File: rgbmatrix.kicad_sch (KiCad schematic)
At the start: 134 parts

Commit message: fked up LEDs :C
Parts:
- D10, D11, D12, D13, D14, D15, D16, D17, D18, D19, D2, D20, D21, D22, D23, D24, D25, D26, D27, D28, D29, D3, D30, D31, D32, D33, D34, D35, D36, D37, D38, D39, D4, D40, D41, D42, D43, D44, D45, D46, D47, D48, D49, D5, D50, D51, D52, D53, D54, D55, D56, D57, D58, D59, D6, D60, D61, D62, D63, D64, D65, D66, D67, D68, D7, D8, D9: footprint LED_SMD:LED_SK6812MINI_PLCC4_3.5x3.5mm_P1.75mm -> reverse:MX_SK6812MINI-E_REV

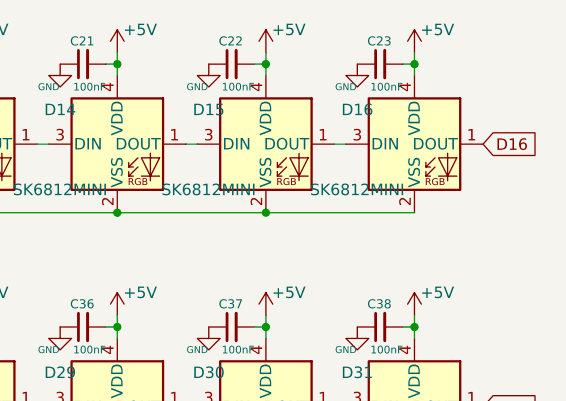
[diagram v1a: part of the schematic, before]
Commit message: pensive
changed LEDs aaaAAAAAAA
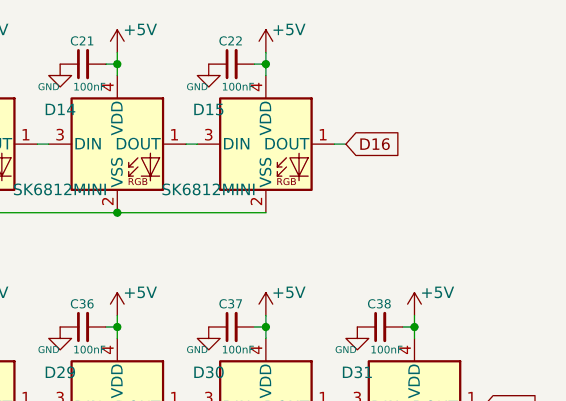
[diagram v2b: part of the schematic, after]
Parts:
- removed C23: 100nF, Capacitor_SMD:C_0805_2012Metric_Pad1.18x1.45mm_HandSolder, symbol Device:C_Small
- removed D16: SK6812MINI, reverse:MX_SK6812MINI-E_REV, symbol LED:SK6812MINI
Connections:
- net D16: now also D15.1 (DOUT)
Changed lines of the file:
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@@
   (junction (at 214.63 105.41) (diameter 0) (color 0 0 0 0)
   )
-  (junction (at 247.65 40.64) (diameter 0) (color 0 0 0 0)
-  )
   (junction (at 66.04 69.85) (diameter 0) (color 0 0 0 0)
   )
@@
   (junction (at 231.14 24.13) (diameter 0) (color 0 0 0 0)
   )
-  (junction (at 264.16 24.13) (diameter 0) (color 0 0 0 0)
-  )
   (junction (at 132.08 96.52) (diameter 0) (color 0 0 0 0)
   )
@@
     (stroke (width 0) (type default) (color 0 0 0 0))
   )
-  (wire (pts (xy 264.16 24.13) (xy 264.16 25.4))
-    (stroke (width 0) (type default) (color 0 0 0 0))
-  )
   (wire (pts (xy 49.53 22.86) (xy 49.53 24.13))
     (stroke (width 0) (type default) (color 0 0 0 0))
@@
     (stroke (width 0) (type default) (color 0 0 0 0))
   )
-  (wire (pts (xy 247.65 40.64) (xy 264.16 40.64))
-    (stroke (width 0) (type default) (color 0 0 0 0))
-  )
   (wire (pts (xy 198.12 80.01) (xy 198.12 81.28))
     (stroke (width 0) (type default) (color 0 0 0 0))
@@
     (stroke (width 0) (type default) (color 0 0 0 0))
   )
-  (wire (pts (xy 264.16 22.86) (xy 264.16 24.13))
-    (stroke (width 0) (type default) (color 0 0 0 0))
-  )
   (wire (pts (xy 148.59 69.85) (xy 165.1 69.85))
     (stroke (width 0) (type default) (color 0 0 0 0))
@@
     (stroke (width 0) (type default) (color 0 0 0 0))
   )
-  (wire (pts (xy 262.89 24.13) (xy 264.16 24.13))
-    (stroke (width 0) (type default) (color 0 0 0 0))
-  )
   (wire (pts (xy 165.1 69.85) (xy 181.61 69.85))
     (stroke (width 0) (type default) (color 0 0 0 0))
@@
     )
   )
-  (global_label "D16" (shape input) (at 271.78 33.02 0) (fields_autoplaced)
+  (global_label "D16" (shape input) (at 256.54 33.02 0) (fields_autoplaced)
     (effects (font (size 1.27 1.27)) (justify left))
-    (property "Intersheet References" "${INTERSHEET_REFS}" (id 0) (at 277.8821 32.9406 0)
+    (property "Intersheet References" "${INTERSHEET_REFS}" (id 0) (at 262.6421 32.9406 0)
       (effects (font (size 1.27 1.27)) (justify left) hide)
     )
@@
     (pin "2")
   )
-  (symbol (lib_id "Device:C_Small") (at 260.35 24.13 90) (unit 1)
-    (in_bom yes) (on_board yes)
-    (property "Reference" "C23" (id 0) (at 261.62 21.59 90)
-      (effects (font (size 1 1)) (justify left))
-    )
-    (property "Value" "100nF" (id 1) (at 262.89 26.67 90)
-      (effects (font (size 0.85 0.85)) (justify left))
-    )
-    (property "Footprint" "Capacitor_SMD:C_0805_2012Metric_Pad1.18x1.45mm_HandSolder" (id 2) (at 260.35 24.13 0)
-      (effects (font (size 1.27 1.27)) hide)
-    )
-    (property "Datasheet" "~" (id 3) (at 260.35 24.13 0)
-      (effects (font (size 1.27 1.27)) hide)
-    )
-    (pin "1")
-    (pin "2")
-  )
   (symbol (lib_id "power:+5V") (at 115.57 104.14 0) (unit 1)
     (in_bom yes) (on_board yes)
@@
     (pin "2")
   )
-  (symbol (lib_id "LED:SK6812MINI") (at 264.16 33.02 0) (unit 1)
-    (in_bom yes) (on_board yes)
-    (property "Reference" "D16" (id 0) (at 257.81 29.21 0))
-    (property "Value" "SK6812MINI" (id 1) (at 257.81 38.1 0))
-    (property "Footprint" "reverse:MX_SK6812MINI-E_REV" (id 2) (at 265.43 40.64 0)
-      (effects (font (size 1.27 1.27)) (justify left top) hide)
-    )
-    (property "Datasheet" "https://cdn-shop.adafruit.com/product-files/2686/SK6812MINI_REV.01-1-2.pdf" (id 3) (at 266.7 42.545 0)
-      (effects (font (size 1.27 1.27)) (justify left top) hide)
-    )
-    (pin "1")
-    (pin "2")
-    (pin "3")
-    (pin "4")
-  )
   (symbol (lib_id "power:+5V") (at 49.53 78.74 0) (unit 1)
     (in_bom yes) (on_board yes)
@@
     (pin "2")
   )
-  (symbol (lib_id "power:+5V") (at 264.16 22.86 0) (unit 1)
-    (in_bom yes) (on_board yes)
-    (property "Reference" "#PWR032" (id 0) (at 264.16 26.67 0)
-      (effects (font (size 1.27 1.27)) hide)
-    )
-    (property "Value" "+5V" (id 1) (at 266.7 20.32 0))
-    (property "Footprint" "" (id 2) (at 264.16 22.86 0)
-      (effects (font (size 1.27 1.27)) hide)
-    )
-    (property "Datasheet" "" (id 3) (at 264.16 22.86 0)
-      (effects (font (size 1.27 1.27)) hide)
-    )
-    (pin "1")
-  )
   (symbol (lib_id "LED:SK6812MINI") (at 165.1 114.3 0) (unit 1)
     (in_bom yes) (on_board yes)
@@
     (pin "2")
   )
-  (symbol (lib_id "power:GND") (at 257.81 24.13 0) (unit 1)
-    (in_bom yes) (on_board yes)
-    (property "Reference" "#PWR0173" (id 0) (at 257.81 30.48 0)
-      (effects (font (size 1.27 1.27)) hide)
-    )
-    (property "Value" "GND" (id 1) (at 256.54 26.67 0)
-      (effects (font (size 0.762 0.762)))
-    )
-    (property "Footprint" "" (id 2) (at 257.81 24.13 0)
-      (effects (font (size 1.27 1.27)) hide)
-    )
-    (property "Datasheet" "" (id 3) (at 257.81 24.13 0)
-      (effects (font (size 1.27 1.27)) hide)
-    )
-    (pin "1")
-  )
   (symbol (lib_id "LED:SK6812MINI") (at 198.12 33.02 0) (unit 1)
